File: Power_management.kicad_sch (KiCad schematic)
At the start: 0 parts

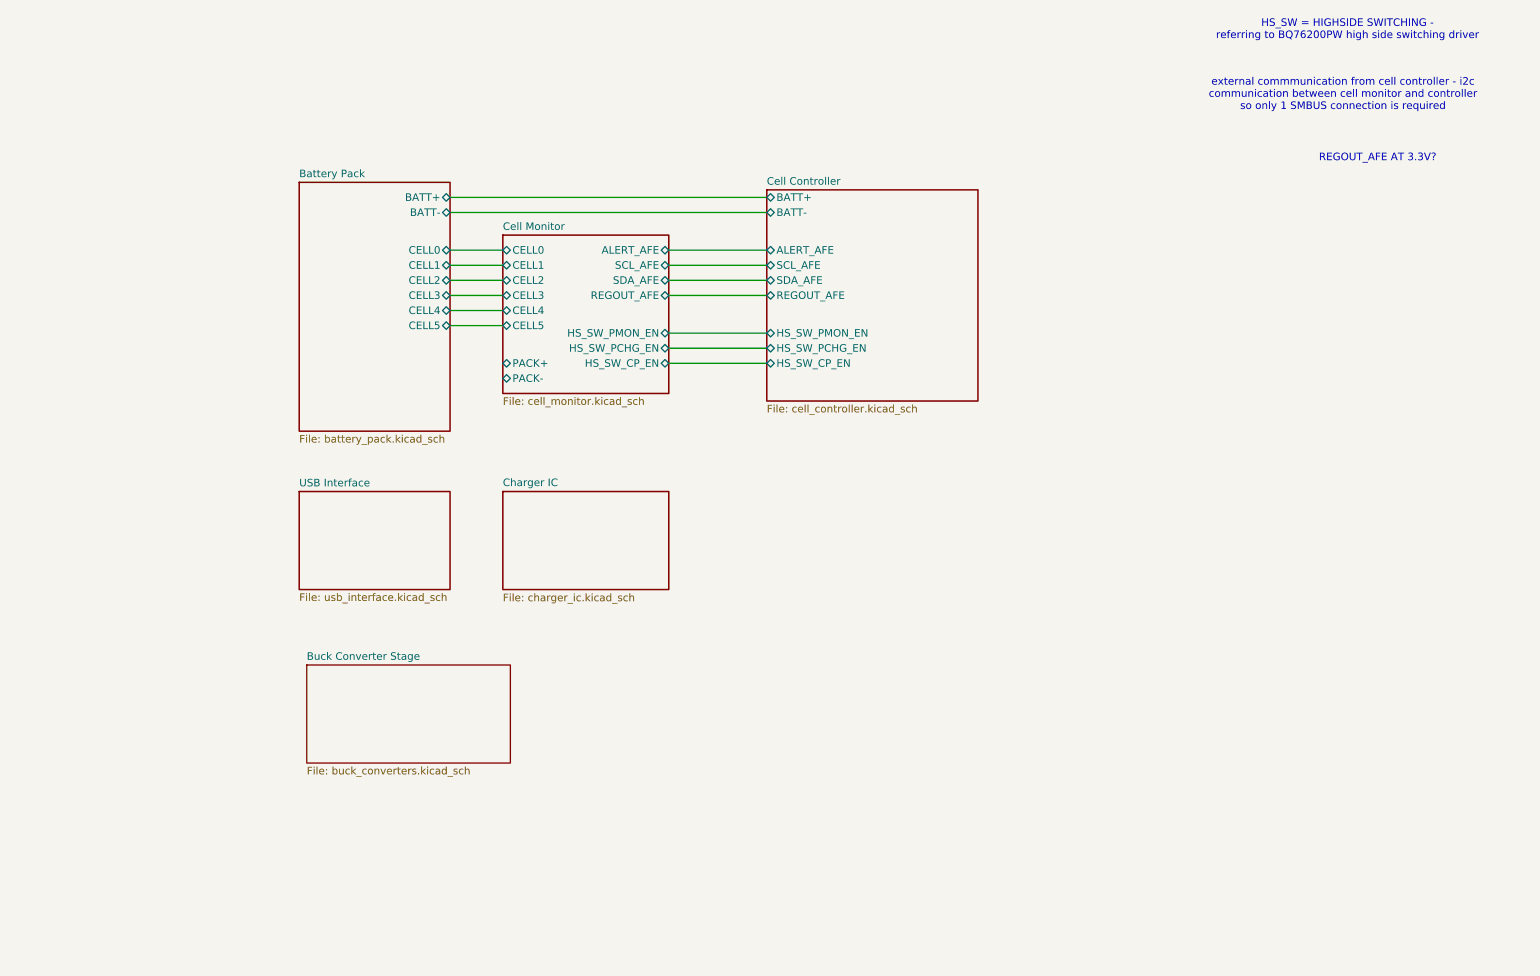
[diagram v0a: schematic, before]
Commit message: structural changes
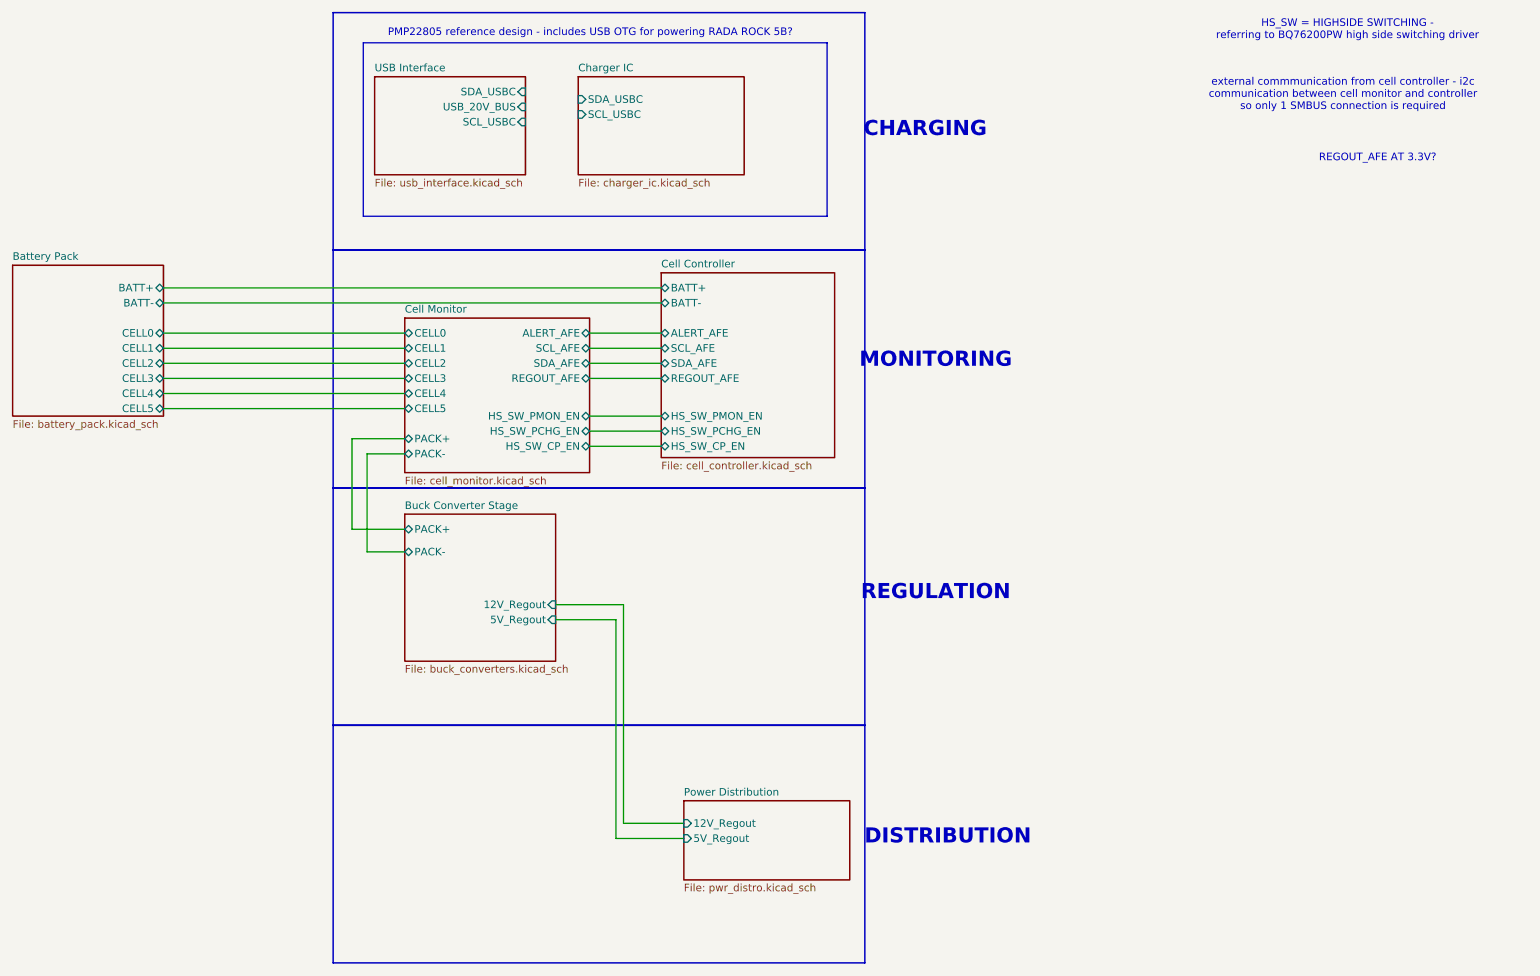
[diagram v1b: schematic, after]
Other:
- added sheet Power Distribution (pwr_distro.kicad_sch)
- sheet Buck Converter Stage ports: added 12V_Regout, 5V_Regout, PACK+, PACK-; removed none
- sheet Charger IC ports: added SCL_USBC, SDA_USBC; removed none
- sheet USB Interface ports: added SCL_USBC, SDA_USBC, USB_20V_BUS; removed none
- note added: "CHARGING"
- note added: "DISTRIBUTION"
- note added: "MONITORING"
- note added: "PMP22805 reference design - includes USB OTG for powering RADA ROCK 5B?"
- note added: "REGULATION"
